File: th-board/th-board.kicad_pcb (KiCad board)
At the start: 2 copper layers, 38.8 x 43 mm, 23 parts, among them J1 Conn_01x02, J2 Conn_01x04, U1 ESP-12F, U2 DHT11, U3 SPX3819M5-L

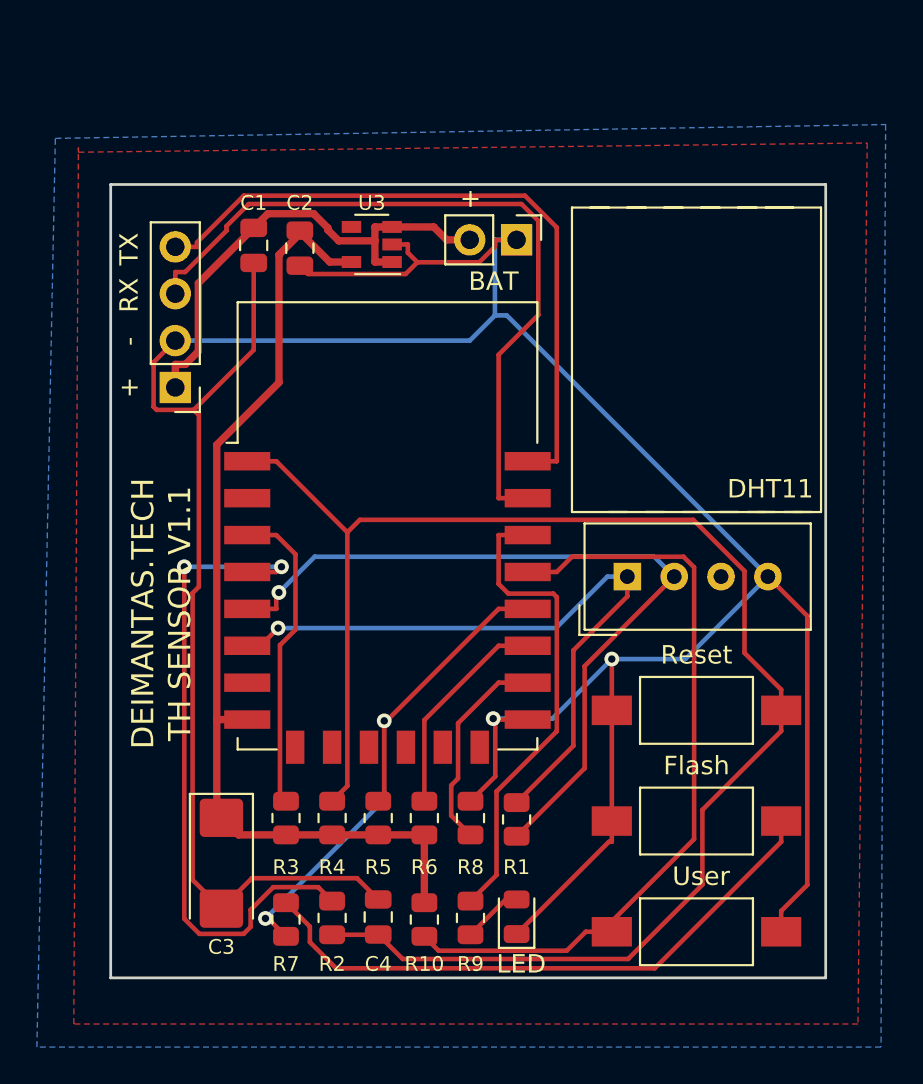
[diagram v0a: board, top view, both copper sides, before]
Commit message: PCB: very small pcb :)
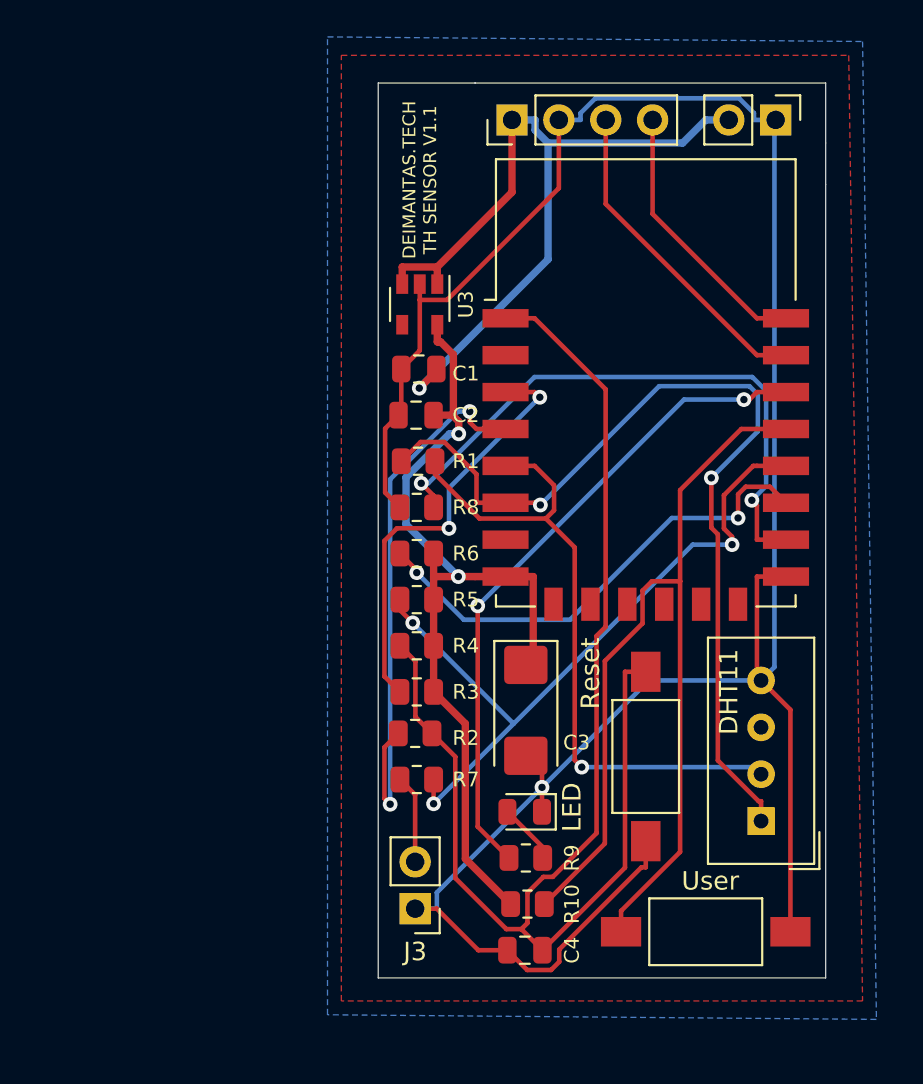
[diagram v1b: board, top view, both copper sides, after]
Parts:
- removed SW_Flash1: SW_Push, Button_Switch_SMD:SW_SPST_FSMSM
- added J3: Conn_01x02, Connector_PinHeader_2.54mm:PinHeader_1x02_P2.54mm_Vertical, F.Cu at (150.5, 110.5)
- moved J2 23.3 mm to (155.8, 67.8), turned to 90 degrees
- moved R1 20.1 mm to (150.7, 86.2), turned to 0 degrees
- moved C3 18.5 mm to (156.5, 99.8)
- moved R8 17.1 mm to (150.6, 88.8), turned to 180 degrees
- moved U1 16.0 mm to (163.0, 82.0)
- moved J1 15.5 mm to (170.0, 67.8)
- moved U2 15.1 mm to (169.2, 105.8), turned to 180 degrees
- moved R6 14.3 mm to (150.6, 91.2), turned to 180 degrees
- moved R5 12.0 mm to (150.6, 93.8), turned to 180 degrees
- moved C1 11.2 mm to (150.7, 81.2), turned to 180 degrees
- moved C2 11.0 mm to (150.6, 83.8), turned to 180 degrees
- moved R2 11.0 mm to (150.5, 101.0), turned to 180 degrees
- moved R4 10.4 mm to (150.6, 96.2), turned to 180 degrees
- moved R7 10.4 mm to (150.6, 103.5), turned to 180 degrees
- moved R3 9.85 mm to (150.6, 98.8), turned to 180 degrees
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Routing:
- net GND: track 174.8 -> 138.4 mm, vias 2 -> 1
- net Net-(J3-Pad2): track 32.8 -> 4.80 mm
- net RX: track 40.4 -> 17.7 mm
- net TX: track 36.9 -> 14.7 mm
- net Net-(R8-Pad1): track 11.3 -> 33.1 mm, vias 0 -> 2
- net Net-(C1-Pad1): track 26.6 -> 44.1 mm, vias 0 -> 1
- net Net-(R6-Pad2): track 11.7 -> 26.6 mm, vias 0 -> 2
- net DHT11_VCC: track 36.9 -> 50.3 mm, vias 1 -> 2
- net USER_BUTTON: track 42.1 -> 53.8 mm
- net RST: track 86.8 -> 76.7 mm
- net Net-(R5-Pad2): track 29.7 -> 39.5 mm, vias 2 -> 3
- net USER_LED: track 26.1 -> 35.9 mm, vias 0 -> 2
- net Net-(R3-Pad2): track 16.9 -> 23.4 mm, vias 0 -> 2
- net Net-(R2-Pad2): track 36.6 -> 30.4 mm
- net DHT11_IO: track 42.8 -> 36.9 mm
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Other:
- board size 38.8 x 43 mm -> 24.2 x 48.5 mm
- board text added: "DEIMANTAS.TECH TH SENSOR V1.1"
- board text removed: "+"
- board text removed: "-"
- board text removed: "BAT"
- board text removed: "DEIMANTAS.TECH"
- board text removed: "Flash"
- board text removed: "RX"
- board text removed: "TH SENSOR V1.1"
- board text removed: "TX"
